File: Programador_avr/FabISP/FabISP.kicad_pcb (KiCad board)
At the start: 2 copper layers, 41 x 19.8 mm, 14 parts, among them IC1 ATTINY44-SSU, M1 Reson., M2 PINHD-1x02-SMD-HEADER, M3 MICRO-USB_1_64

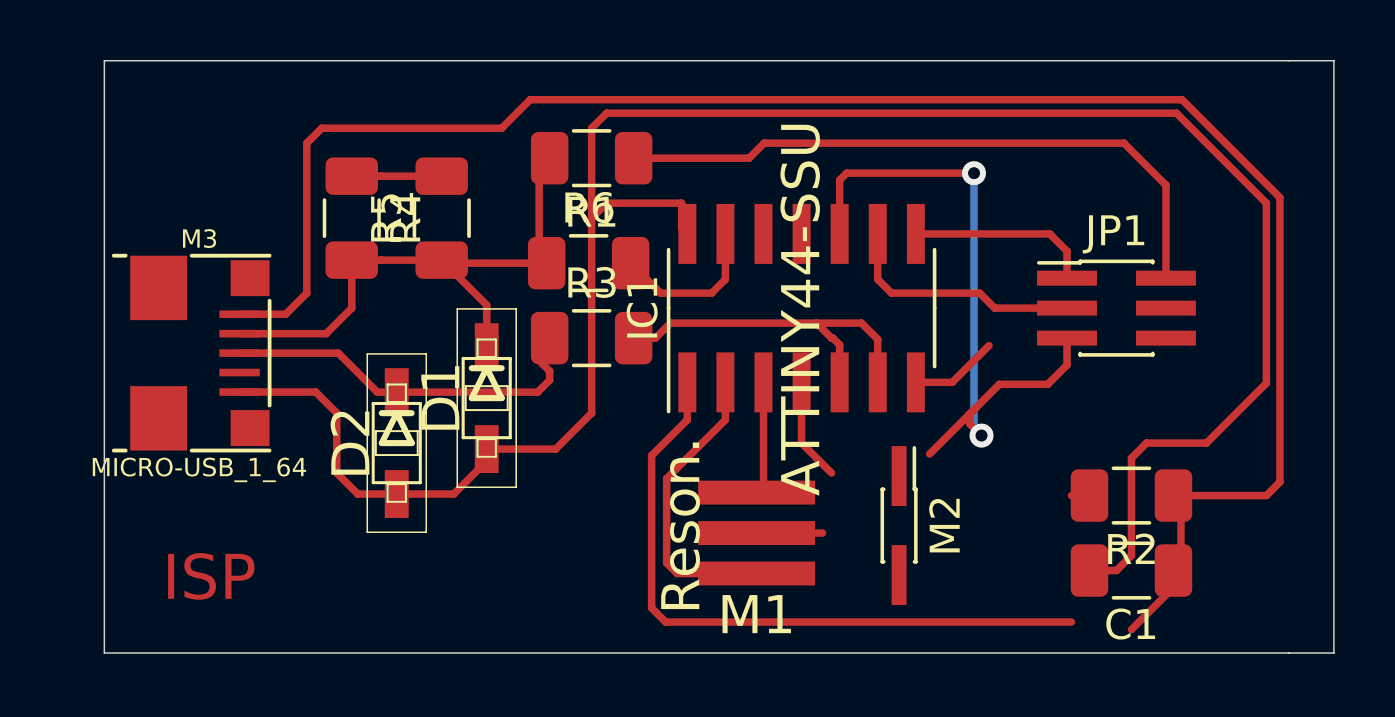
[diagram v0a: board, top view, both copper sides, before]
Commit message: Correcciones
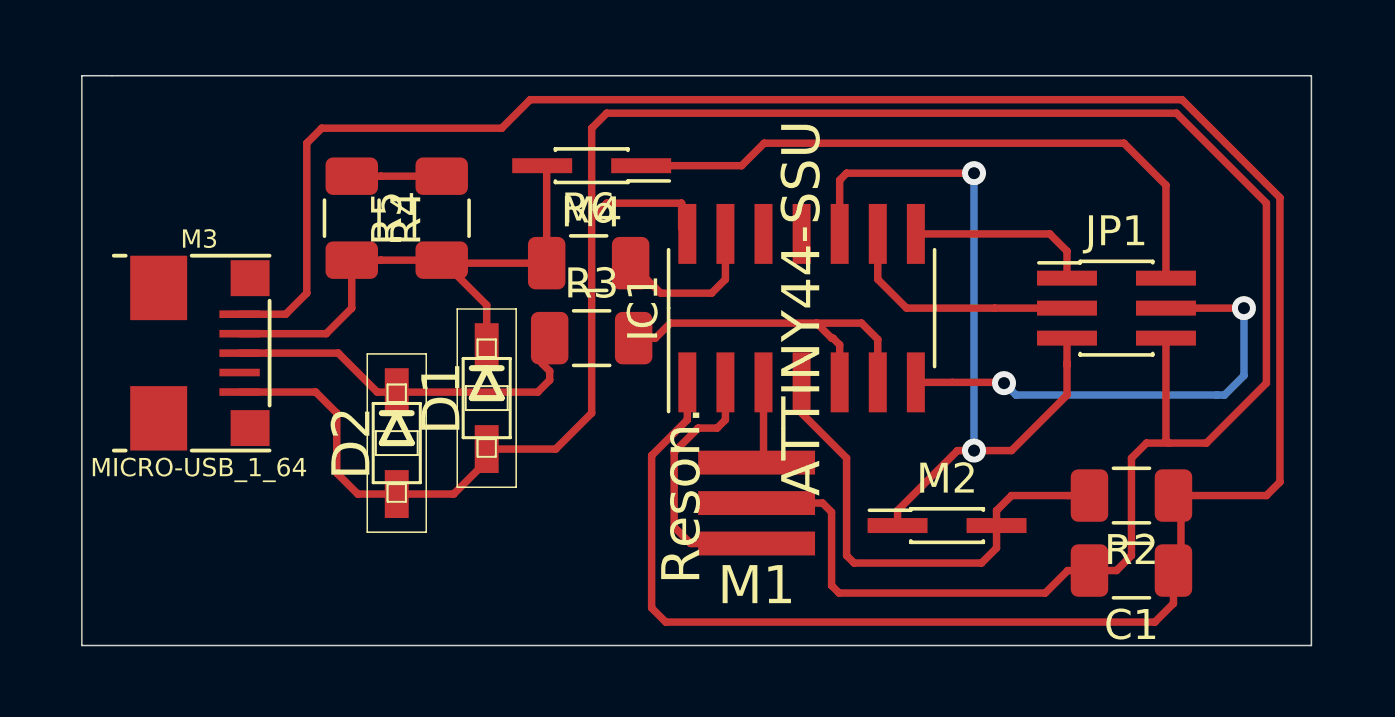
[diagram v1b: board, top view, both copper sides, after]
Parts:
- removed R1: 0, Resistor_SMD:R_1206_3216Metric
- added M4: PINHD-1x02-SMD-HEADER, Connector_PinHeader_1.00mm:PinHeader_2x01_P1.00mm_Vertical_SMD, F.Cu at (61.0, 54.0)
- moved M2 1.60 mm to (72.8, 66.0), turned to 0 degrees
- moved M1 1.00 mm to (66.5, 65.2)
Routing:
- net GND: track 72.3 -> 87.7 mm
- net /MOSI: track 2.95 -> 16.2 mm, vias 0 -> 2
- net /PB3: track 3.79 -> 16.6 mm
- net VCC: track 82.3 -> 84.7 mm
- net /RST: track 23.1 -> 25.3 mm
- net /XTAL1: track 9.98 -> 8.88 mm
- net /XTAL2: track 3.77 -> 2.77 mm
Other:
- board size 41 x 19.8 mm -> 41 x 19 mm
- board text added: "ISP_AVR_Programmer"
- board text removed: "ISP"
